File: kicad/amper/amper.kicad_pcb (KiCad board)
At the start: 2 copper layers, 91.4 x 91.4 mm, 47 parts, among them J1 Conn_01x05, J2 Conn_01x02, J3 Conn_01x15, J4 Conn_01x10, J5 Conn_01x10, Q1 FDS9435A, Q2 FDS9435A, SW1 SW_Push, SW2 SW_Push, SW3 SW_Push, SW4 SW_Push, U1 114-87-308-41-134161, U2 HDSM-441B, U3 HDSM-441B, U4 HDSM-441B, U5 TM1637, U6 ATtiny40-SU

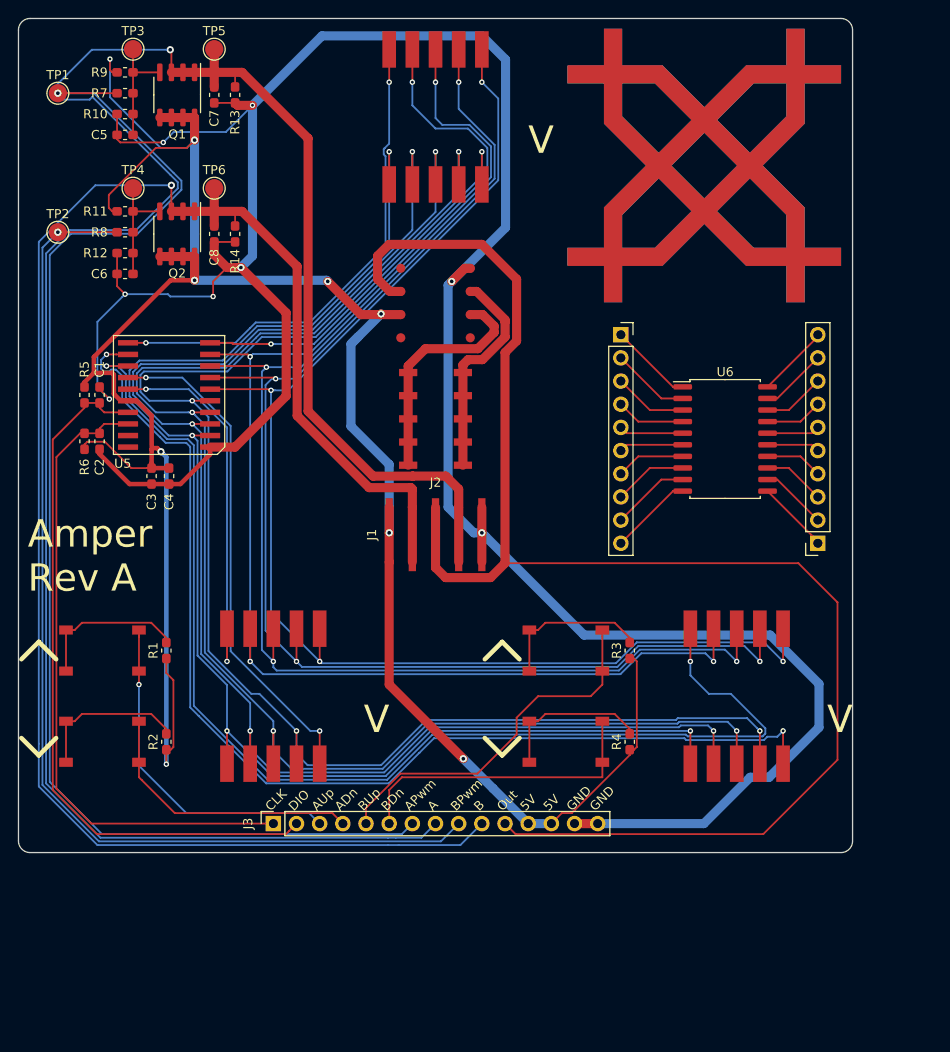
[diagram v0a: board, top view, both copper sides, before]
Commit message: Reannotated everything
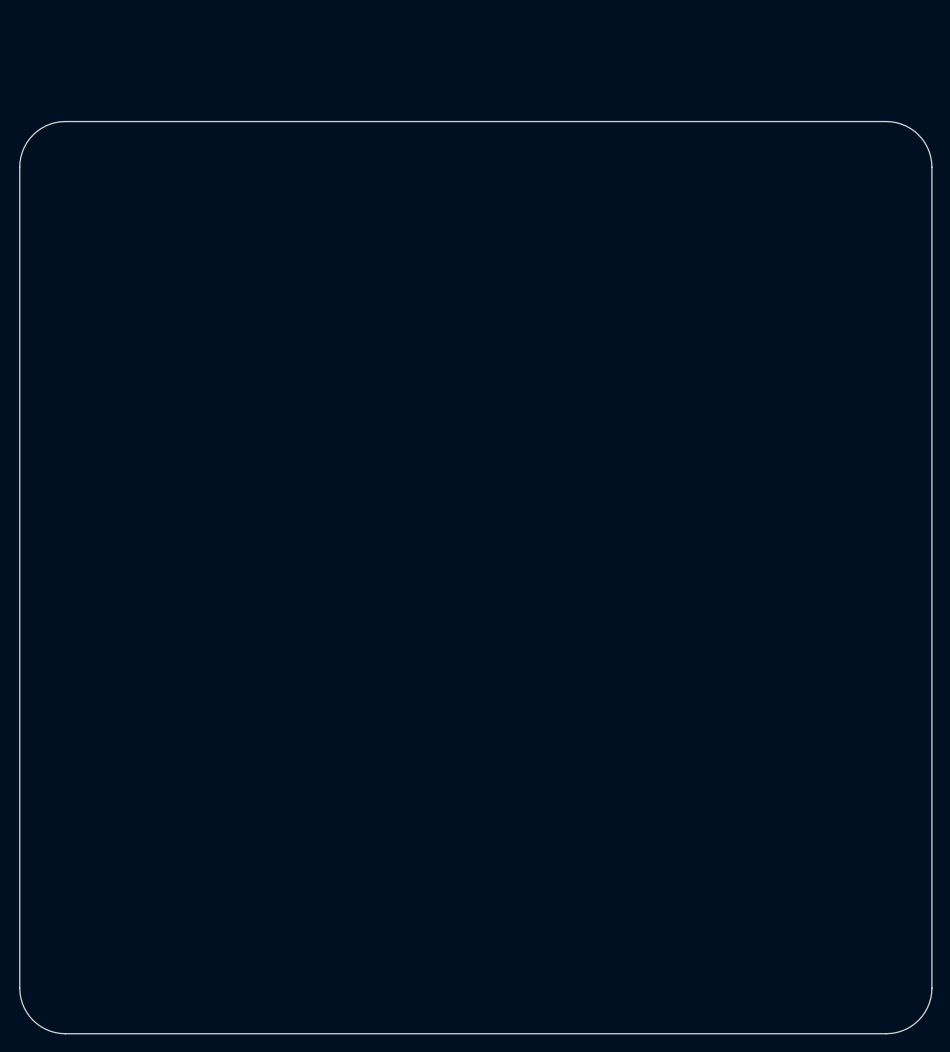
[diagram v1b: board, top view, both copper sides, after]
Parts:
- removed C1, C2: 100pF, Capacitor_SMD:C_0603_1608Metric_Pad1.05x0.95mm_HandSolder
- removed C3: 100nF, Capacitor_SMD:C_0603_1608Metric_Pad1.05x0.95mm_HandSolder
- removed C4: 10uF, Capacitor_SMD:C_0603_1608Metric_Pad1.05x0.95mm_HandSolder
- removed C5, C6, C7, C8: 1u, Capacitor_SMD:C_0603_1608Metric_Pad1.05x0.95mm_HandSolder
- removed J1: Conn_01x05, amper:2.54_2x5_col_ganged
- removed J2: Conn_01x02, amper:2.54_2x5_row_ganged
- removed J3: Conn_01x15, Connector_PinSocket_2.54mm:PinSocket_1x15_P2.54mm_Vertical
- removed J4, J5: Conn_01x10, Connector_PinSocket_2.54mm:PinSocket_1x10_P2.54mm_Vertical
- removed Q1, Q2: FDS9435A, Package_SO:SOIC-8_3.9x4.9mm_P1.27mm
- removed R1, R2, R3, R4, R5, R6: 10K, Resistor_SMD:R_0603_1608Metric_Pad1.05x0.95mm_HandSolder
- removed R10, R12: 40k, Resistor_SMD:R_0603_1608Metric_Pad1.05x0.95mm_HandSolder
- removed R11, R9: 25k, Resistor_SMD:R_0603_1608Metric_Pad1.05x0.95mm_HandSolder
- removed R13, R14: 100K, Resistor_SMD:R_0603_1608Metric_Pad1.05x0.95mm_HandSolder
- removed R7, R8: 60k, Resistor_SMD:R_0603_1608Metric_Pad1.05x0.95mm_HandSolder
- removed SW1, SW2, SW3, SW4: SW_Push, amper:K2-1157SP-I4SW-01
- removed TP1, TP2, TP3, TP4, TP5, TP6: TestPoint, TestPoint:TestPoint_Pad_D2.0mm
- removed U1: 114-87-308-41-134161, amper:114-87-308-41-134161
- removed U2, U3, U4: HDSM-441B, amper:SLS0392FB4A1GD
- removed U5: TM1637, amper:TM1637
- removed U6: ATtiny40-SU, Package_SO:SOIC-20W_7.5x12.8mm_P1.27mm
- removed svg2mod (x2): G***, amper:pcb_logo
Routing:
- net GND: track 302.6 -> 0.00 mm, vias 8 -> 0
- net +5V: track 272.9 -> 0.00 mm, vias 9 -> 0
- net /SourceA: track 239.8 -> 0.00 mm, vias 1 -> 0
- net /SourceB: track 194.2 -> 0.00 mm, vias 1 -> 0
- net /SEG4: track 166.4 -> 0.00 mm, vias 4 -> 0
- net /AmpOut: track 165.8 -> 0.00 mm
- net /SEG3: track 163.5 -> 0.00 mm, vias 4 -> 0
- net /SEG2: track 161.2 -> 0.00 mm, vias 4 -> 0
- net /SEG1: track 157.7 -> 0.00 mm, vias 4 -> 0
- net /SEG8: track 151.3 -> 0.00 mm, vias 4 -> 0
- net /SEG7: track 151.0 -> 0.00 mm, vias 4 -> 0
- net /SEG6: track 149.2 -> 0.00 mm, vias 4 -> 0
- net /SEG5: track 148.1 -> 0.00 mm, vias 4 -> 0
- net /SourceAPWM: track 142.8 -> 0.00 mm, vias 1 -> 0
- net /SourceBDigit1: track 130.2 -> 0.00 mm, vias 2 -> 0
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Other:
- board size 91.4 x 91.4 mm -> 100 x 100 mm
- board text removed: "5V"
- board text removed: "A"
- board text removed: "ADn"
- board text removed: "APwm"
- board text removed: "AUp"
- board text removed: "Amper Rev A"
- board text removed: "B"
- board text removed: "BDn"
- board text removed: "BPwm"
- board text removed: "BUp"
- board text removed: "CLK"
- board text removed: "DIO"
- board text removed: "GND"
- board text removed: "Out"
- board text removed: "V"
